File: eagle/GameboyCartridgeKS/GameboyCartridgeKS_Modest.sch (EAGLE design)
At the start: 20 parts, among them IC2 MEGA64-A, Y1 16MHz max

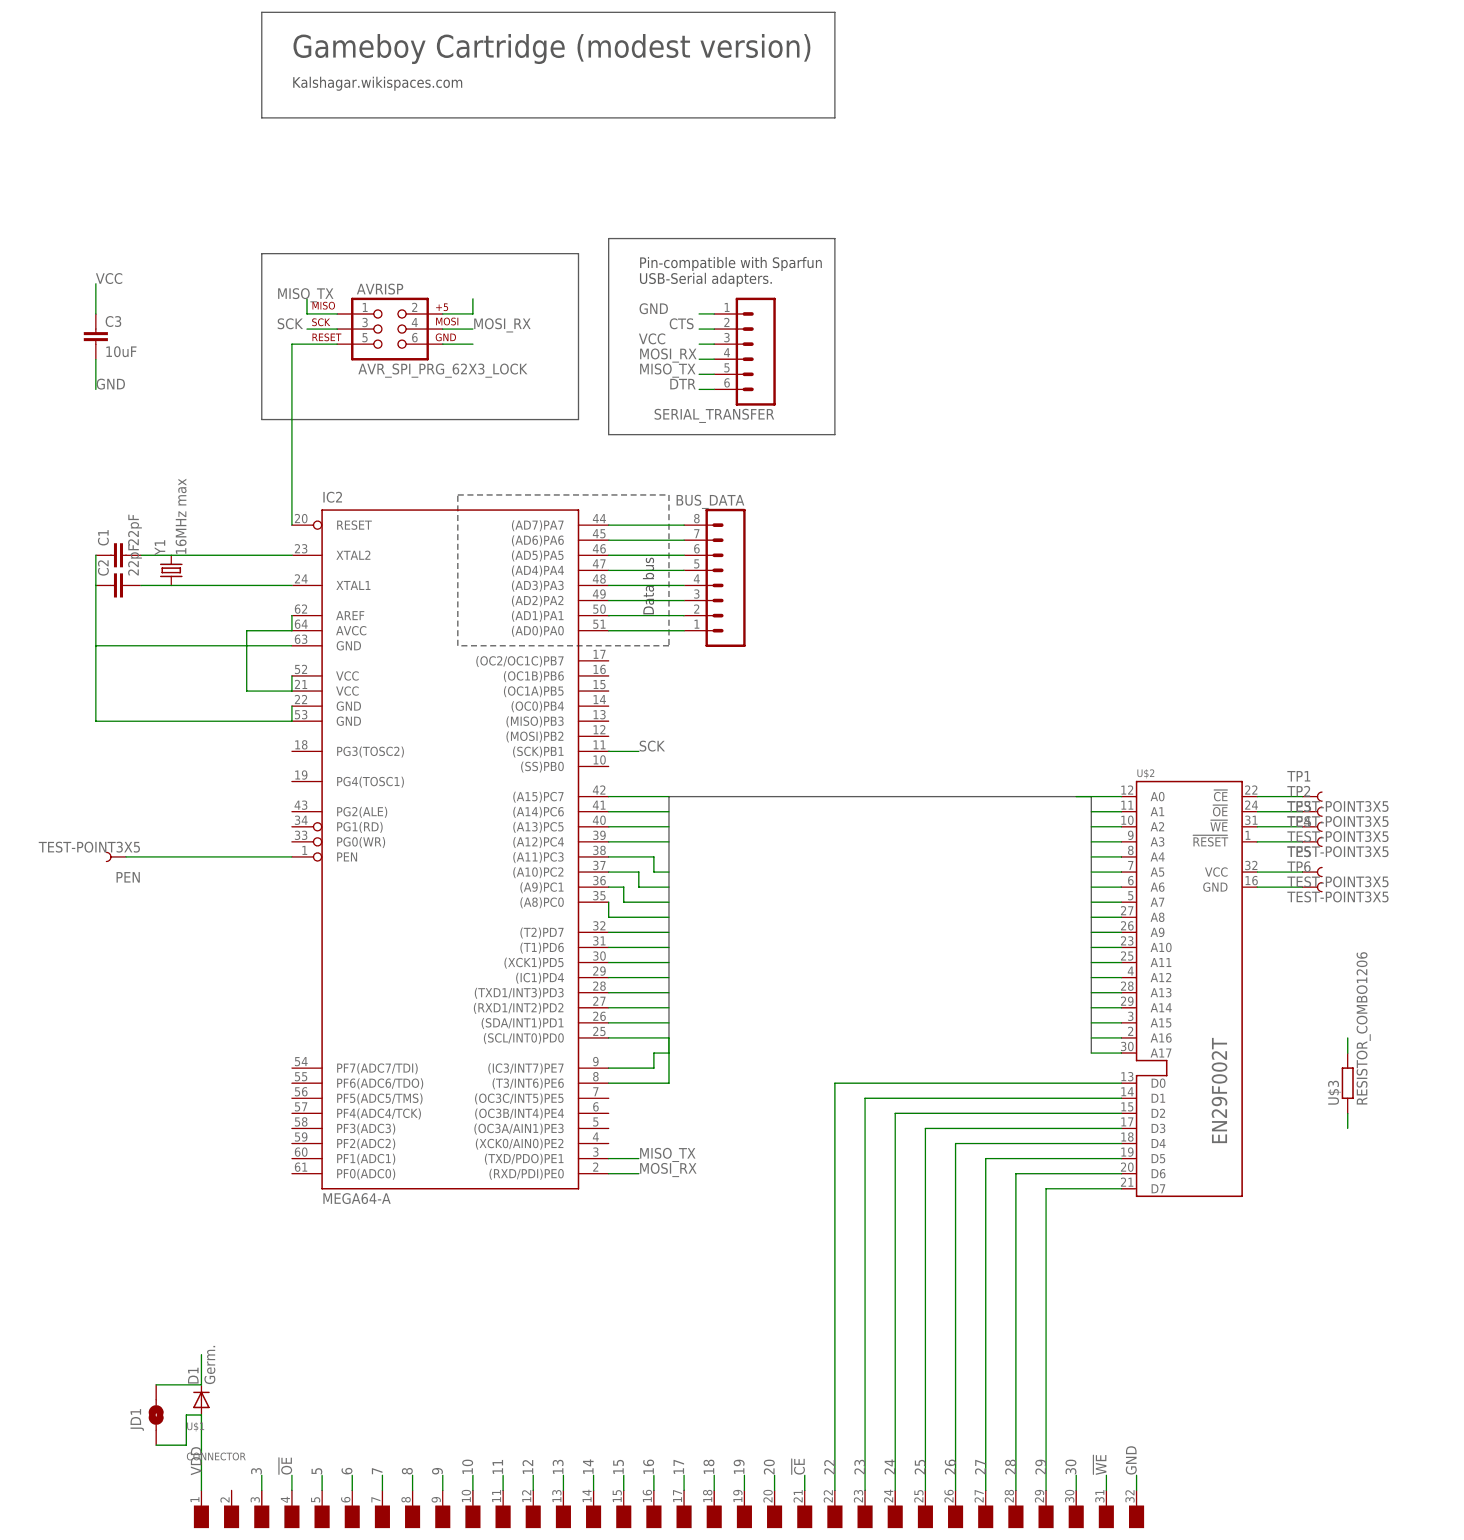
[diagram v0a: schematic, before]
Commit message: Modest beta before wiring
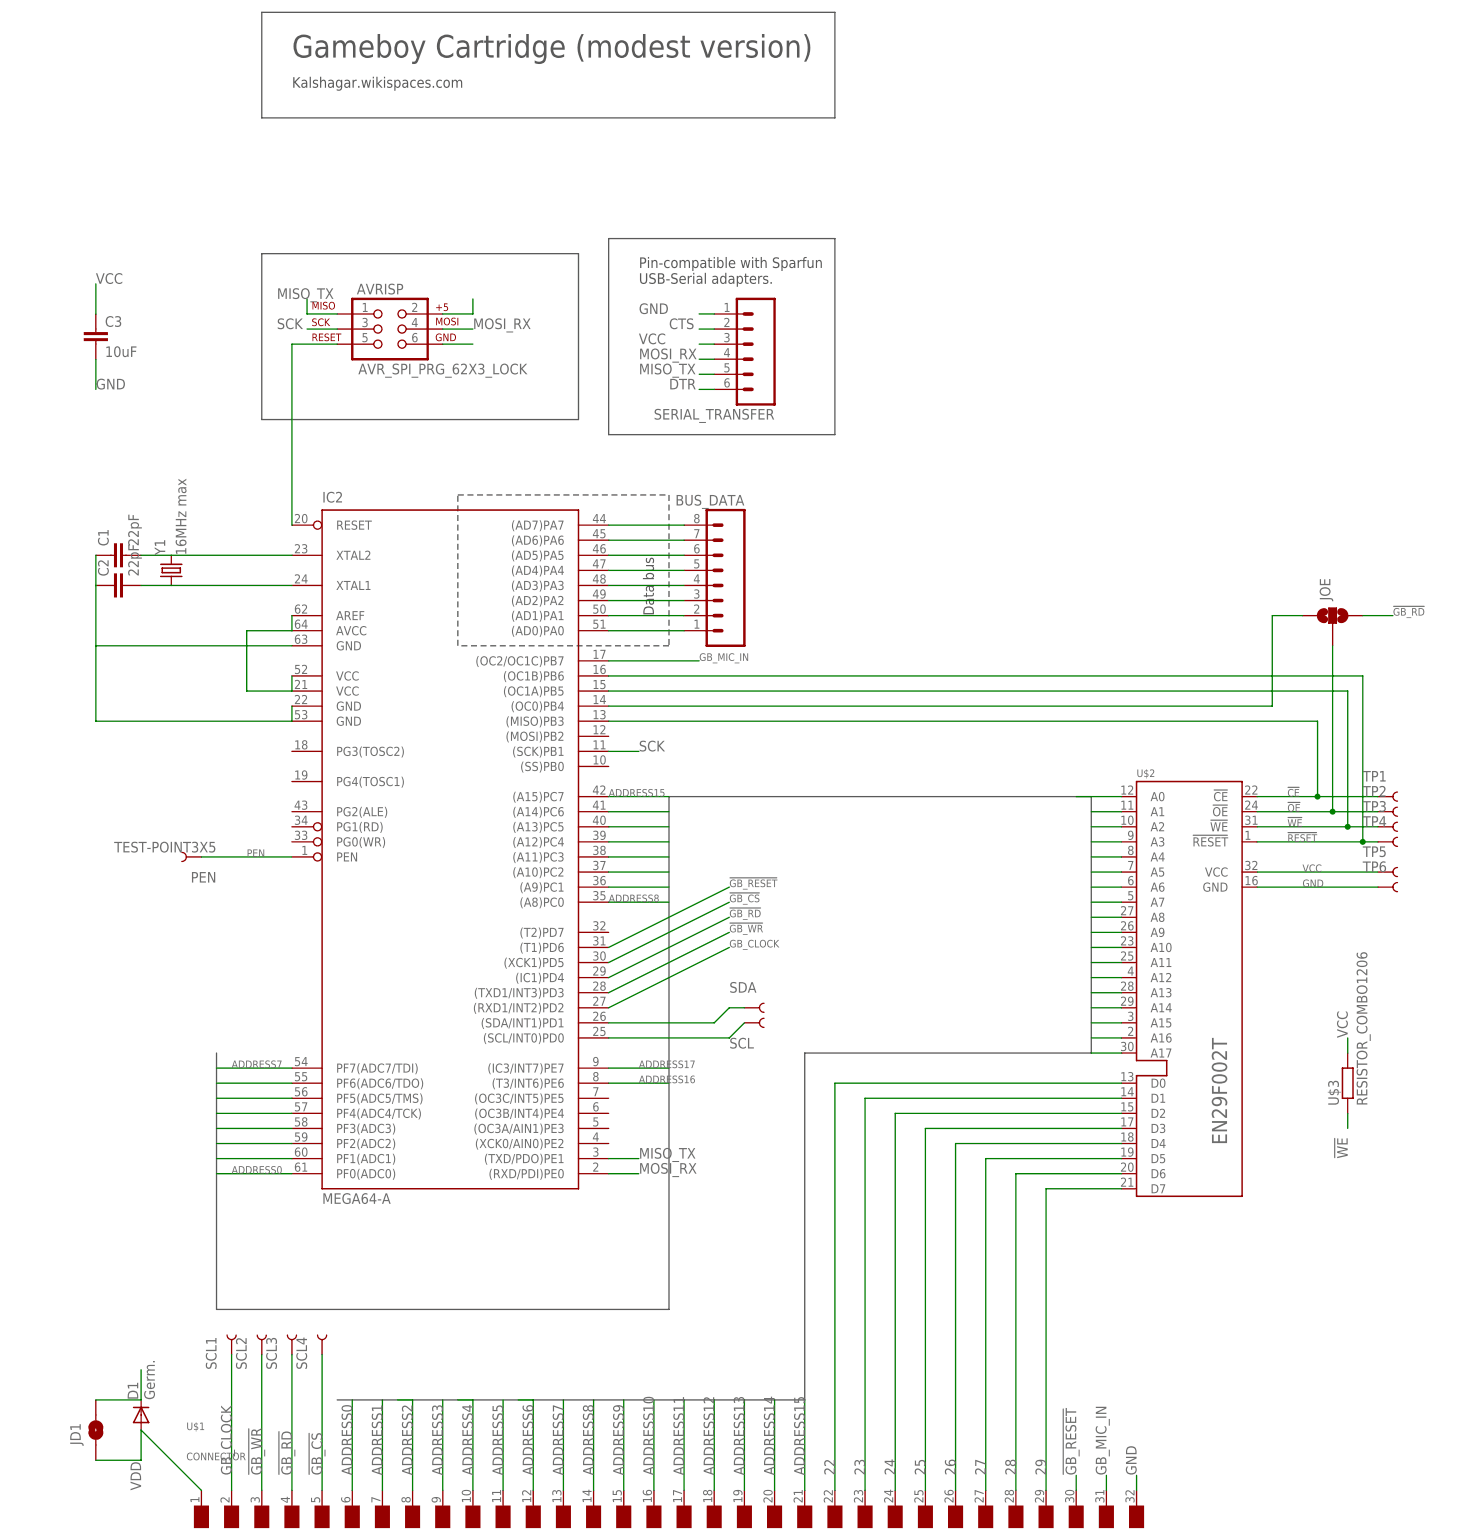
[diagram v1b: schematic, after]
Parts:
- added JOE: JUMPER-PAD-3-NOYES_SILK, SparkFun-Passives:JUMPER-PAD-3-NOYES_SILK
- added SCL, SCL1, SCL2, SCL3, SCL4, SDA: TEST-POINT3X5, SparkFun-Passives:TEST-POINT3X5
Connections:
- removed net 10: U$1.A4
- removed net 11: U$1.A5
- removed net 12: U$1.A6
- removed net 13: U$1.A7
- removed net 14: U$1.A8
- removed net 15: U$1.A9
- removed net 16: U$1.A10
- removed net 17: U$1.A11
- removed net 18: U$1.A12
- removed net 19: U$1.A13
- removed net 20: U$1.A14
- removed net 3: U$1./WR
- removed net 30: U$1./RS
- removed net 5: U$1./RCS
- removed net 6: U$1.A0
- removed net 7: U$1.A1
- removed net 8: U$1.A2
- removed net 9: U$1.A3
- new net !GB_CS: IC2.(XCK1)PD5, SCL4.1, U$1./RCS
- new net !GB_RD: IC2.(IC1)PD4, JOE.3, SCL3.1, U$1./RD
- new net !GB_RESET: IC2.(T1)PD6, U$1./RS
- new net !GB_WR: IC2.(TXD1/INT3)PD3, SCL2.1, U$1./WR
- new net GB_CLOCK: IC2.(RXD1/INT2)PD2, SCL1.1, U$1.NC
- new net GB_MIC_IN: IC2.(OC2/OC1C)PB7, U$1.VIN
- new net N$1: IC2.(SDA/INT1)PD1, SDA.1
- new net N$5: IC2.(SCL/INT0)PD0, SCL.1
- new net N$7: IC2.(OC0)PB4, JOE.1
- net !CE: now also IC2.(MISO)PB3; no longer U$1.A15
- net !OE: now also JOE.2; no longer U$1./RD
- net !RESET: now also IC2.(OC1B)PB6
- net !WE: now also IC2.(OC1A)PB5; no longer U$1.VIN
- net ADDRESS0: now also IC2.PF0(ADC0), U$1.A0; no longer IC2.(SCL/INT0)PD0
- net ADDRESS1: now also IC2.PF1(ADC1), U$1.A1; no longer IC2.(SDA/INT1)PD1
- net ADDRESS10: now also U$1.A10
- net ADDRESS11: now also U$1.A11
- net ADDRESS12: now also U$1.A12
- net ADDRESS13: now also U$1.A13
- net ADDRESS14: now also U$1.A14
- net ADDRESS15: now also U$1.A15
- net ADDRESS2: now also IC2.PF2(ADC2), U$1.A2; no longer IC2.(RXD1/INT2)PD2
- net ADDRESS3: now also IC2.PF3(ADC3), U$1.A3; no longer IC2.(TXD1/INT3)PD3
- net ADDRESS4: now also IC2.PF4(ADC4/TCK), U$1.A4; no longer IC2.(IC1)PD4
- net ADDRESS5: now also IC2.PF5(ADC5/TMS), U$1.A5; no longer IC2.(XCK1)PD5
- net ADDRESS6: now also IC2.PF6(ADC6/TDO), U$1.A6; no longer IC2.(T1)PD6
- net ADDRESS7: now also IC2.PF7(ADC7/TDI), U$1.A7; no longer IC2.(T2)PD7
- net ADDRESS8: now also U$1.A8
- net ADDRESS9: now also U$1.A9
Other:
- moved on the sheet: D1, JD1, PEN, TP1, TP2, TP3, TP4, TP5, TP6
